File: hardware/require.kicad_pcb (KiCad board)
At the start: 6 copper layers, 68 x 26 mm, 180 parts, among them J800 Molex 105164-0001, Q110 LN235N3T5G, Q840 LMBT3904DW1T1G, U100 RK3308, U200 SY8089AAC, U220 PAM2305CGFADJ, U230 PAM2305CGFADJ, U250 PAM2305CGFADJ, U260 NCP707CMX180TCG, U300 DDR3_FBGA96, U400 EMMC_BGA_153, U500 ap6255, U830 ATECC608A-MAHDA, Y100 24MHz,12pF,10ppm, Y520 37.4MHz,9pF,10ppm

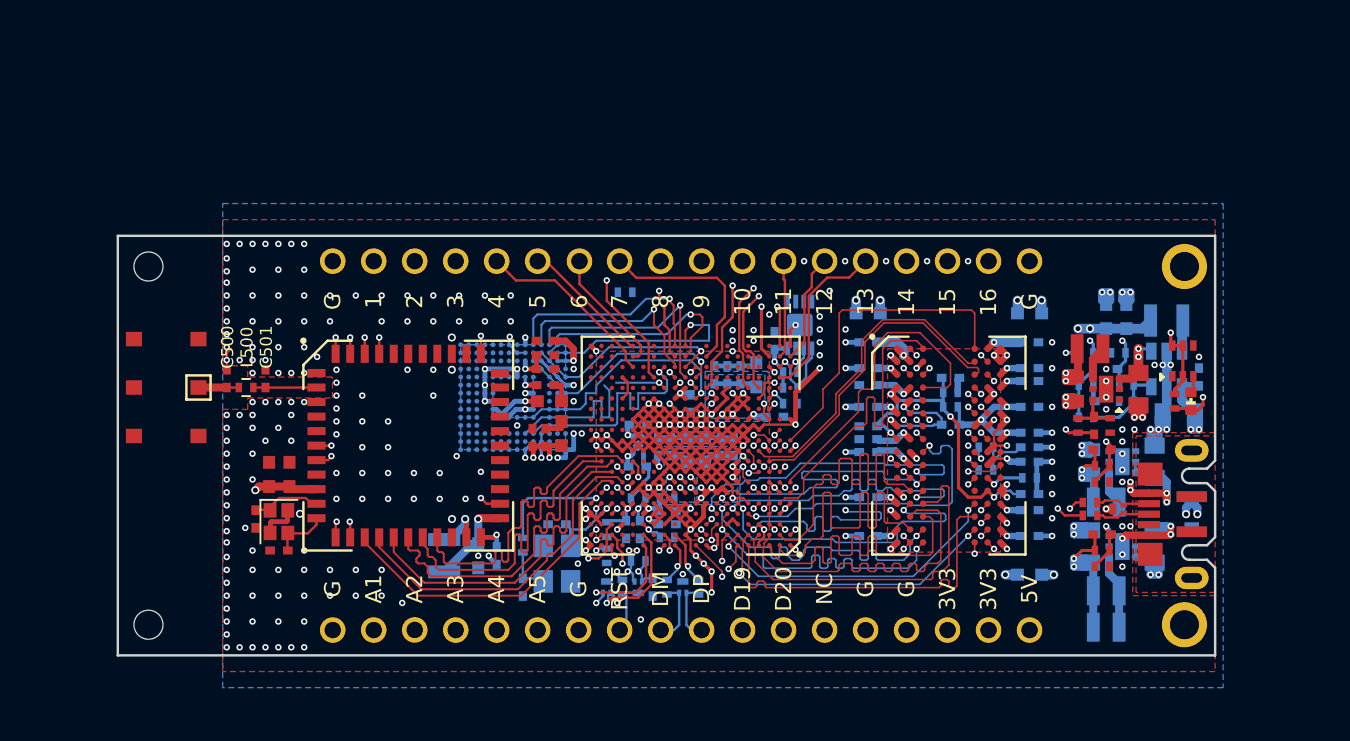
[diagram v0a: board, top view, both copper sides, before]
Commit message: wip
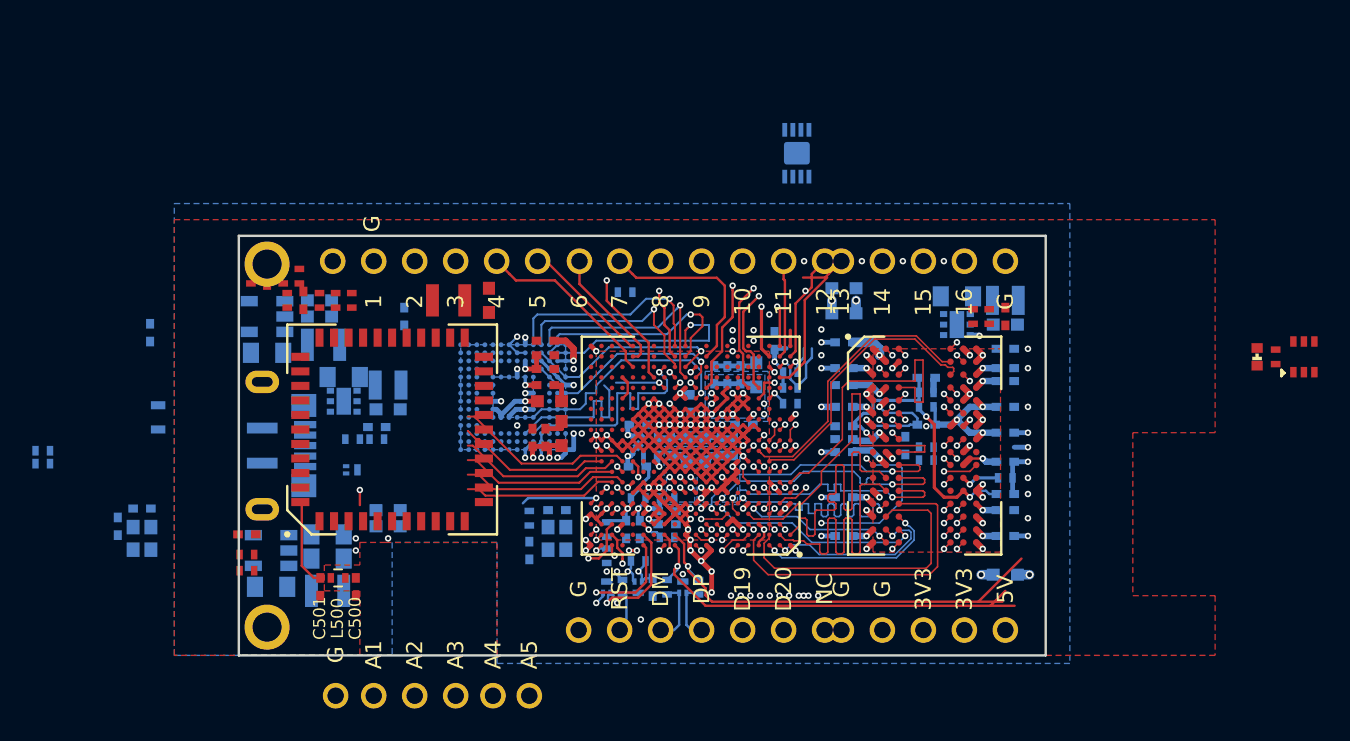
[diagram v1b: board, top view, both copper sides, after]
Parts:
- removed A500: AH104N2450D1-T, require:ANT_AH104N
- removed H1, H2: MountingHole, require:MTG_1.8mm_2.4mm_NPL
- removed L251: 2.2u, require:L_0806
- added C254: 10u,10V, require:C_0805, B.Cu at (42.5, 72.0)
- C202, C210, C540, L540, R201, R202, R203, R210, R211, R212, R213: moved to F.Cu
- C222, C231, C233, C510, C511, C520, C521, D800, J800, L230, R222, R223, R800, R801, U230, Y520: moved to B.Cu
- L250: footprint require:L_0806 -> require:L_1008
- U250: value PAM2305CGFADJ -> SY8089AAC; footprint require:U-DFN2020-6 -> require:SOT-23-5
- Y100: footprint Crystals:Crystal_SMD_3225-4pin_3.2x2.5mm -> Crystals:Crystal_SMD_2016-4pin_2.0x1.6mm
- moved C200 65.1 mm to (31.5, 58.0)
- moved R800 65.0 mm to (24.9, 66.1), turned to 0 degrees
- moved R801 65.0 mm to (24.9, 65.3), turned to 0 degrees
- moved R802 64.3 mm to (32.0, 63.2)
- moved J800 60.6 mm to (37.0, 65.0)
- moved H3 56.9 mm to (38.8, 53.8)
- moved H4 56.9 mm to (38.8, 76.2)
- moved C201 56.6 mm to (38.8, 59.2), turned to 0 degrees
- moved U200 55.8 mm to (38.8, 57.0), turned to 180 degrees
- moved C251 54.8 mm to (39.0, 73.8), turned to 0 degrees
- moved R203 54.8 mm to (37.8, 54.5), turned to 90 degrees
- moved C202 53.6 mm to (38.8, 54.5), turned to 270 degrees
- moved R252 53.0 mm to (37.5, 72.8)
- moved R253 53.0 mm to (37.5, 71.8)
- moved C252 53.0 mm to (37.5, 70.5)
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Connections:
- U250 pad 1: Net-(U250-Pad1) -> +5V
- U250 pad 2: +5V -> GND
- U250 pad 3: +5V -> Net-(L250-Pad1)
- U250 pad 4: Net-(L250-Pad1) -> +5V
- U250 pad 5: GND -> Net-(C252-Pad2)
- U300 pad A3: /ddr/DDR_D4 -> /ddr/DDR_D5
- U300 pad C8: /ddr/DDR_D5 -> /ddr/DDR_D4
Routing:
- net GND: track 281.7 -> 228.1 mm, vias 293 -> 115
- net +1V0C: track 48.6 -> 18.1 mm, vias 9 -> 6
- net /rk3308-io/USB_HOST_DP: track 3.41 -> 28.0 mm
- net /rk3308-io/USB_HOST_DM: track 2.62 -> 26.4 mm
- net +5V: track 21.7 -> 0.00 mm, vias 10 -> 0
- net /power/CORE_DVS: track 21.3 -> 0.46 mm, vias 2 -> 1
- net /rk3308-io/BT_WAKE_HOST: track 20.4 -> 0.00 mm, vias 3 -> 0
- net +3V3: track 51.3 -> 32.2 mm, vias 18 -> 12
- net /ddr/DDR_CLKN: track 20.9 -> 5.42 mm
- net /ddr/DDR_CLKP: track 20.7 -> 5.32 mm
- net /LED: track 35.2 -> 22.1 mm, vias 2 -> 1
- net /ddr/DDR_RESET: track 22.6 -> 9.53 mm, vias 3 -> 2
- net /rk3308-io/SDIO_D2: track 21.2 -> 9.48 mm
- net /rk3308-io/SDIO_D0: track 21.1 -> 9.50 mm
- net /rk3308-io/SDIO_CMD: track 21.4 -> 9.80 mm
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- removed copper zone on F.Cu, net /SHIELD
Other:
- board size 68 x 26 mm -> 50 x 26 mm

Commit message: wip
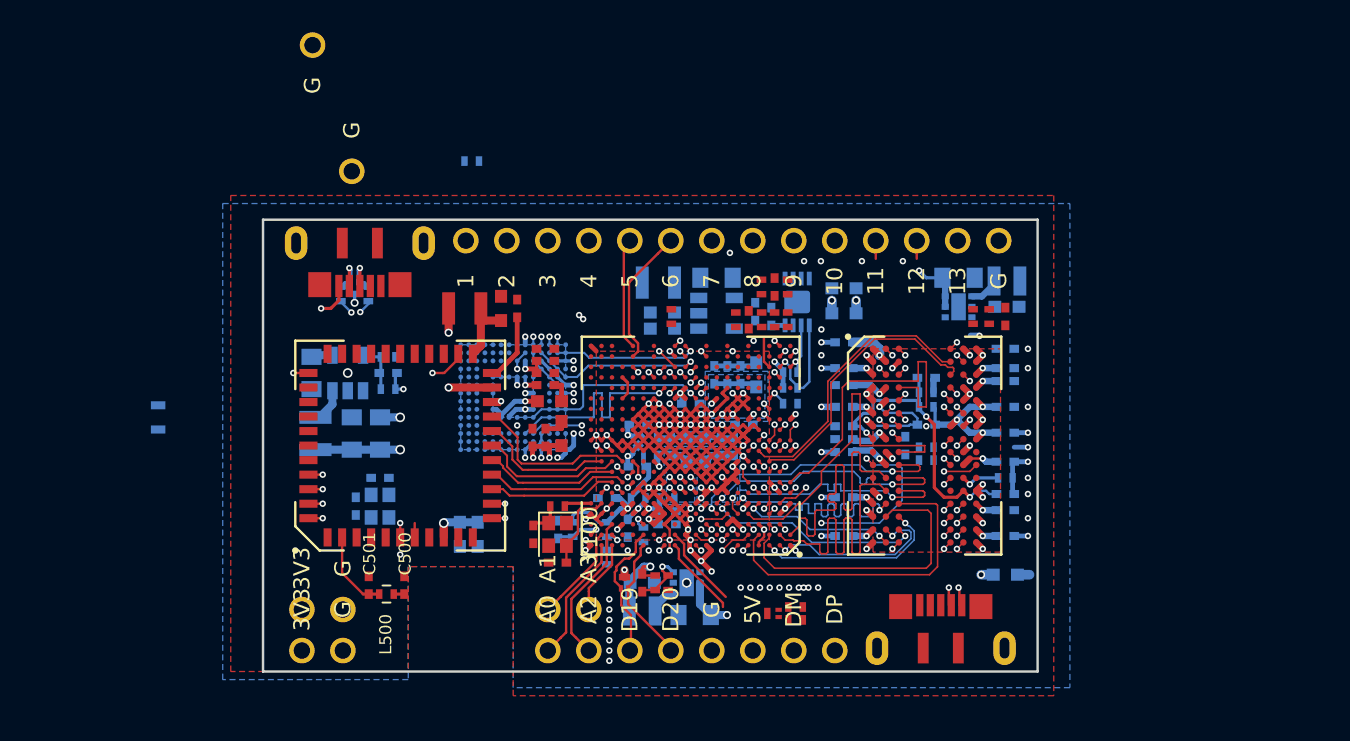
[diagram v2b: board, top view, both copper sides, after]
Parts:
- removed D840: LED, require:LED_0402
- removed H3, H4: MountingHole_Pad, require:MTG_1.8mm_2.4mm_PL
- removed the J800 at (37.0, 65.0)
- removed LP13: NC, require:OVAL_PIN
- removed LP6: A5, require:OVAL_PIN
- removed LP8: RST, require:OVAL_PIN
- removed Q110: LN235N3T5G, require:SOT-883
- removed Q840: LMBT3904DW1T1G, require:SOT-363_SC-70-6
- removed R111: 10k, require:R_0402
- removed R840: 470R, require:R_0402
- removed RP15: 14, require:OVAL_PIN
- removed RP16: 15, require:OVAL_PIN
- removed RP17: 16, require:OVAL_PIN
- added J800: Molex 105164-0001, require:USB_Micro-B_Molex-105164-0001, F.Cu at (44.5, 51.0)
- added J800: Molex 105164-0001, require:USB_Micro-B_Molex-105164-0001, F.Cu at (80.5, 79.0)
- C100, C101, C222, C530, D810, D820, R100, R222, R223, R810, R811, Y100: moved to F.Cu
- C252, R252, R253: moved to B.Cu
- LP2: value A1 -> A0
- LP3: value A2 -> A1
- LP4: value A3 -> A2
- LP5: value A4 -> A3
- moved LP15 43.5 mm to (44.0, 48.0)
- moved LP17 41.1 mm to (40.9, 77.7)
- moved LP16 38.5 mm to (40.9, 75.2)
- moved C200 37.5 mm to (69.0, 56.7), turned to 270 degrees
- moved LP14 30.9 mm to (43.5, 77.7)
- moved R203 30.2 mm to (67.8, 57.2)
- moved C202 30.0 mm to (68.6, 57.2), turned to 90 degrees
- moved R202 29.8 mm to (69.4, 57.2), turned to 90 degrees
- moved R210 29.4 mm to (69.4, 55.2), turned to 90 degrees
- moved C210 29.2 mm to (70.2, 55.2)
- moved R211 29.0 mm to (71.0, 55.2), turned to 90 degrees
- moved C201 28.2 mm to (66.6, 54.6), turned to 180 degrees
- moved U200 27.9 mm to (66.6, 56.8), turned to 0 degrees
- moved R212 27.2 mm to (70.2, 57.2), turned to 270 degrees
- moved R213 27.0 mm to (71.0, 57.2)
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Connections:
- net /EMMC_D0 renamed /emmc/EMMC_D0
- net /KEY renamed Net-(U100-PadT1)
- net /rk3308-io/PCM_CLK renamed Net-(U100-PadF18)
- net /rk3308-io/PCM_IN renamed Net-(U100-PadH14)
- net /rk3308-io/PCM_OUT renamed Net-(U100-PadH15)
- net /rk3308-io/PCM_SYNC renamed Net-(U100-PadJ15)
- net /rk3308-power/RESET_1V8 renamed Net-(C110-Pad1)
- LP2 pad 1: /rk3308-io/A1 -> /rk3308-io/A0
- LP3 pad 1: /rk3308-io/A2 -> /rk3308-io/A1
- LP4 pad 1: /rk3308-io/A3 -> /rk3308-io/A2
- LP5 pad 1: /rk3308-io/A4 -> /rk3308-io/A3
- R400 pad 1: /emmc/EMMC_CLK1 -> Net-(R400-Pad1)
- R400 pad 2: /emmc/EMMC_CLK -> Net-(R400-Pad2)
- R700 pad 2: /rk3308-io/A0 -> /rk3308-io/A4
- R701 pad 1: /rk3308-io/A0 -> /rk3308-io/A4
- R800 pad 1: Net-(D800-Pad1) -> Net-(D800-Pad2)
- R801 pad 1: Net-(D800-Pad2) -> Net-(D800-Pad1)
- U100 pad R4: /rk3308-io/D14 -> Net-(U100-PadR4)
- U100 pad T4: /rk3308-io/D16 -> Net-(U100-PadT4)
- U100 pad T5: /rk3308-io/D15 -> Net-(U100-PadT5)
- U100 pad W3: /LED -> Net-(U100-PadW3)
- U400 pad A8: /emmc/EMMC_D7 -> Net-(U400-PadA8)
- U400 pad B7: /emmc/EMMC_D7 -> Net-(U400-PadB7)
- U400 pad C7: Net-(U400-PadC7) -> /emmc/EMMC_D7
- U400 pad K1: /emmc/EMMC_CLK1 -> /emmc/EMMC_CLK
- U400 pad K2: /emmc/EMMC_CLK1 -> /emmc/EMMC_CLK
- U400 pad K3: /emmc/EMMC_CLK1 -> /emmc/EMMC_CLK
- U400 pad M6: /emmc/EMMC_CLK1 -> /emmc/EMMC_CLK
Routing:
- net +3V3: track 32.2 -> 56.2 mm, vias 12 -> 14
- net /rk3308-io/USB_HOST_DP: track 28.0 -> 5.15 mm, vias 1 -> 0
- net /LED: track 22.1 -> 0.00 mm, vias 1 -> 0
- net /rk3308-io/BT_REG_ON: track 8.77 -> 30.8 mm, vias 1 -> 2
- net /rk3308-io/D16: track 22.0 -> 0.00 mm, vias 1 -> 0
- net /rk3308-io/USB_HOST_DM: track 26.4 -> 5.06 mm, vias 1 -> 0
- net /rk3308-io/D15: track 19.9 -> 0.00 mm, vias 1 -> 0
- net /rk3308-io/BT_WAKE_HOST: track 0.00 -> 17.4 mm, vias 0 -> 2
- net /rk3308-io/D14: track 15.5 -> 0.00 mm, vias 2 -> 0
- net /rk3308-io/D20: track 19.6 -> 8.01 mm, vias 2 -> 0
- net /rk3308-io/A1: track 17.6 -> 6.01 mm, vias 1 -> 0
- net /emmc/EMMC_CLK: track 3.14 -> 13.7 mm
- net +5V: track 0.00 -> 10.3 mm, vias 0 -> 3
- net /rk3308-io/A5: track 10.0 -> 0.00 mm, vias 1 -> 0
- net /emmc/EMMC_CLK1: track 9.77 -> 0.00 mm
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- added copper zone on In4.Cu, net +5V
- removed copper zone on In3.Cu, net +5V
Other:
- board size 50 x 26 mm -> 48 x 28 mm
